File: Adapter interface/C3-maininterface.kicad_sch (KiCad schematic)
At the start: 4 parts, among them J1 SFM-120-02-L-DH, J2 SFM-120-02-L-DH

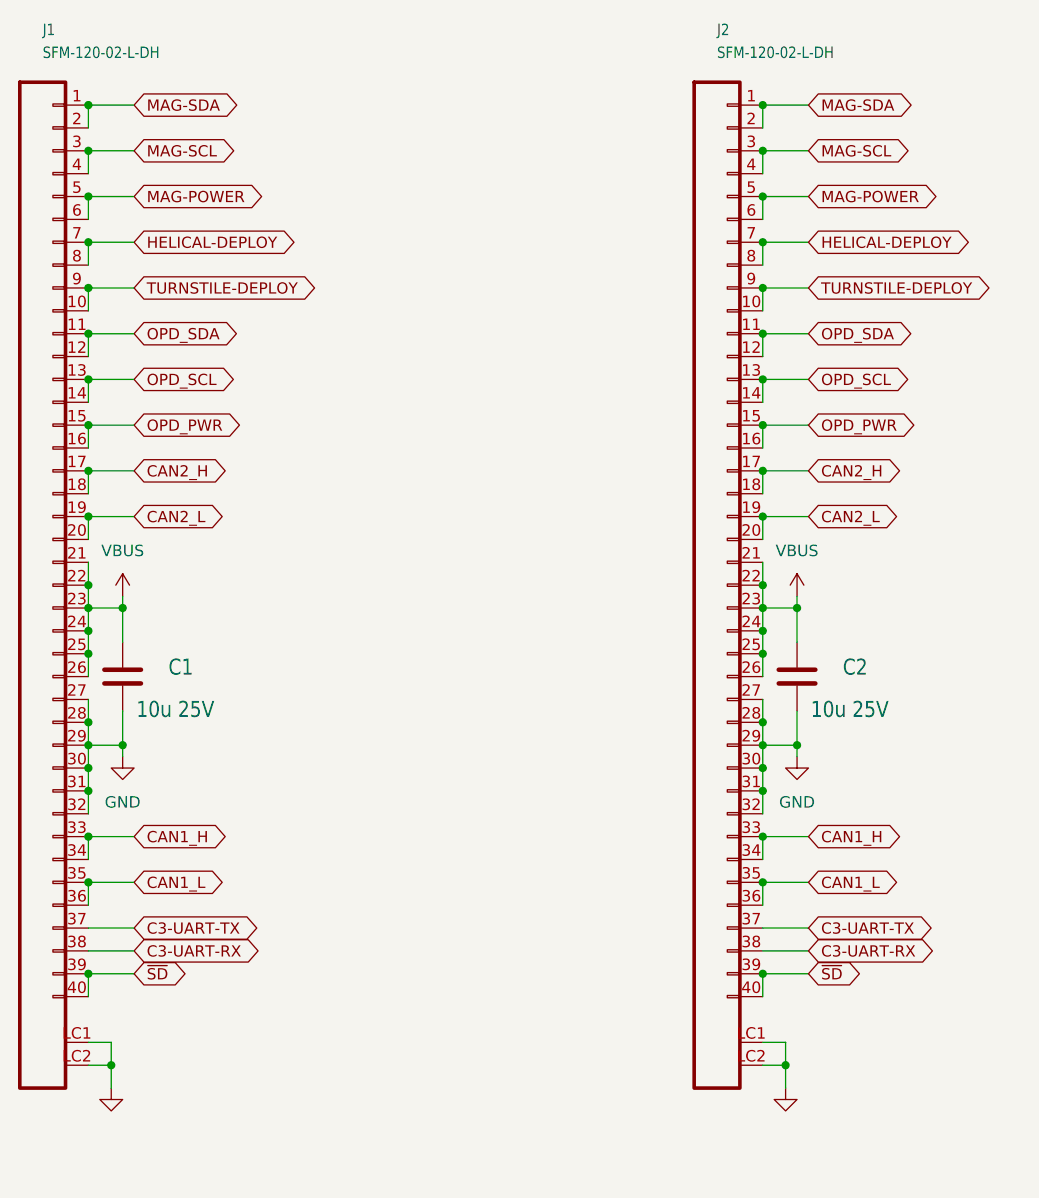
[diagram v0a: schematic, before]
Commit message: New connectors
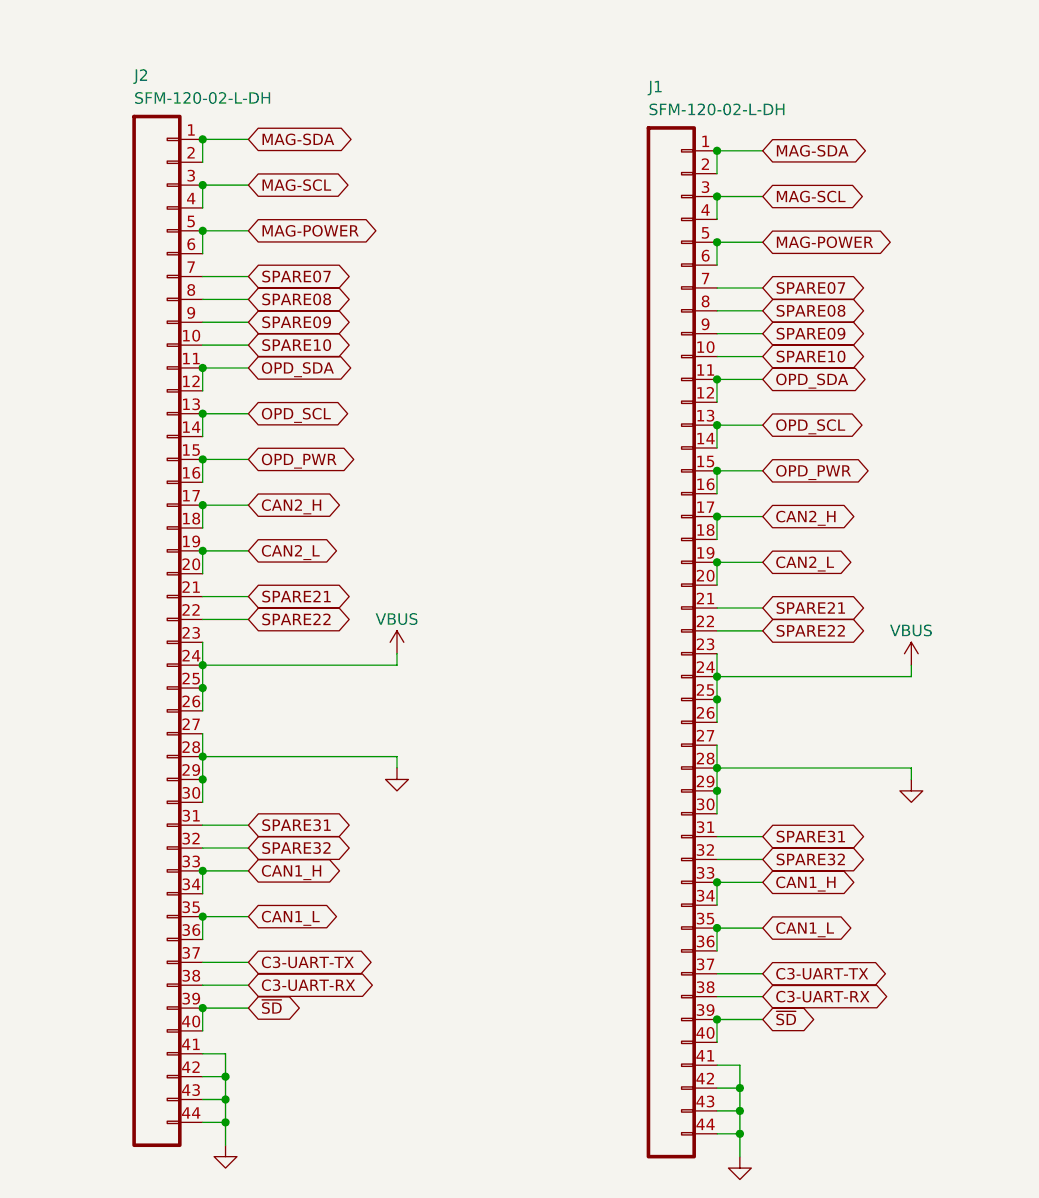
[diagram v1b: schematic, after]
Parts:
- removed C1, C2: 10u 25V, Capacitor_SMD:C_1206_3216Metric, symbol Device:C
- removed J1, J2: SFM-120-02-L-DH, oresat-connectors:J-SAMTEC-SFM-120-X1-XXX-D, symbol oresat-connectors:J-SAMTEC-SFM-120-X1-XXX-D
- added J1, J2: SFM-120-02-L-DH, oresat-connectors:SFM-120-02-X-DH, symbol oresat-connectors:SFM-120-02-X-DH
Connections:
- net C3-UART-RX: now also J1.38, J2.38
- net C3-UART-TX: now also J1.37, J2.37
- net CAN1_H: now also J1.33, J1.34, J2.33, J2.34
- net CAN1_L: now also J1.35, J1.36, J2.35, J2.36
- net CAN2_H: now also J1.17, J1.18, J2.17, J2.18
- net CAN2_L: now also J1.19, J1.20, J2.19, J2.20
- net GND: now also J1.27, J1.28, J1.29, J1.30, J1.41, J1.42, J1.43, J1.44, J2.27, J2.28, J2.29, J2.30, J2.41, J2.42, J2.43, J2.44
- net MAG-POWER: now also J1.5, J1.6, J2.5, J2.6
- net MAG-SCL: now also J1.3, J1.4, J2.3, J2.4
- net MAG-SDA: now also J1.1, J1.2, J2.1, J2.2
- net OPD_PWR: now also J1.15, J1.16, J2.15, J2.16
- net OPD_SCL: now also J1.13, J1.14, J2.13, J2.14
- net OPD_SDA: now also J1.11, J1.12, J2.11, J2.12
- net VBUS: now also J1.23, J1.24, J1.25, J1.26, J2.23, J2.24, J2.25, J2.26
- net ~{SD}: now also J1.39, J1.40, J2.39, J2.40
- new net SPARE07: J1.7, J2.7
- new net SPARE08: J1.8, J2.8
- new net SPARE09: J1.9, J2.9
- new net SPARE10: J1.10, J2.10
- new net SPARE21: J1.21, J2.21
- new net SPARE22: J1.22, J2.22
- new net SPARE31: J1.31, J2.31
- new net SPARE32: J1.32, J2.32
